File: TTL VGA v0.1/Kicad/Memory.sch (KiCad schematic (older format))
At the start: 16 parts, among them U10 UM61512A, U11 74LS245, U12 74LS374, U13 74LS245, U14 74LS245, U6 G22V10, U7 G22V10, U8 74LS139, U9 UM61512A

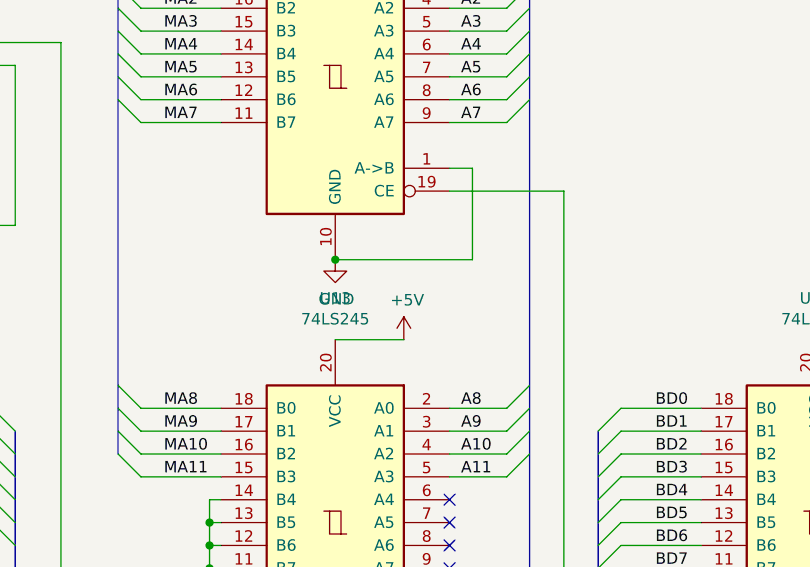
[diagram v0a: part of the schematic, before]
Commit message: update kicad
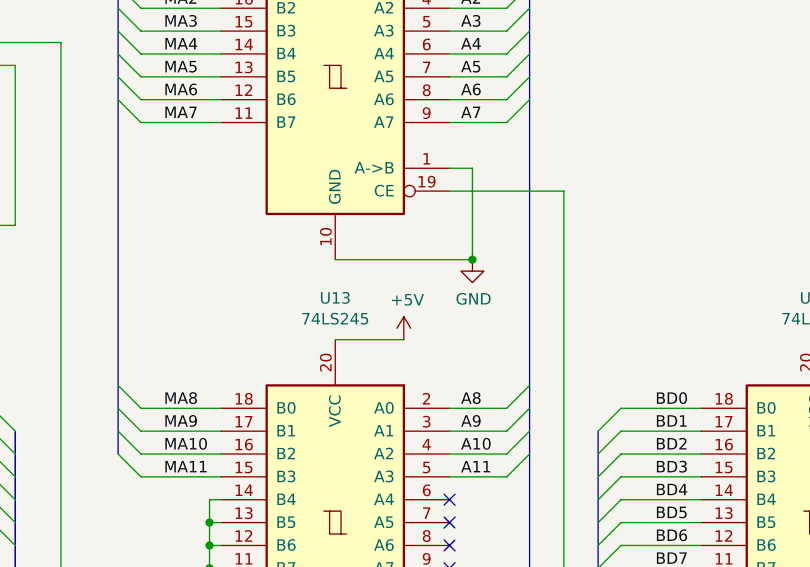
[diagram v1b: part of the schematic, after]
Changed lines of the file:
@@
 L power:GND #PWR022
 U 1 1 5E68F558
-P 4350 5750
-F 0 "#PWR022" H 4350 5500 50  0001 C CNN
-F 1 "GND" H 4355 5577 50  0000 C CNN
-F 2 "" H 4350 5750 50  0001 C CNN
-F 3 "" H 4350 5750 50  0001 C CNN
-	1    4350 5750
+P 4950 5750
+F 0 "#PWR022" H 4950 5500 50  0001 C CNN
+F 1 "GND" H 4955 5577 50  0000 C CNN
+F 2 "" H 4950 5750 50  0001 C CNN
+F 3 "" H 4950 5750 50  0001 C CNN
+	1    4950 5750
 	1    0    0    -1
 $EndComp
@@
 Wire Wire Line
 	4950 5750 4350 5750
-Connection ~ 4350 5750
 Wire Wire Line
 	4850 7300 4950 7300
@@
 $EndComp
 NoConn ~ 2600 7100
-Wire Bus Line
-	2950 6500 2950 8100
-Wire Bus Line
-	11700 2650 11700 4000
-Wire Bus Line
-	7350 5900 7350 7000
-Wire Bus Line
-	5500 6500 5500 8250
-Wire Bus Line
-	1250 4950 1250 8250
-Wire Bus Line
-	9250 2650 9250 5900
-Wire Bus Line
-	3400 3700 3400 6600
-Wire Bus Line
-	9550 1100 9550 4600
-Wire Bus Line
-	5200 1100 5200 8100
-Wire Bus Line
-	7100 1100 7100 4600
 Text Notes 7250 1800 0    50   ~ 0
 A16 and A17 are swapped on the 74LS139.\n(but it is wired like this on the perf board)\nThis will fail when using more VRAM chips.\nFix by swapping outputs in U7 (WinCUPL).
+Wire Bus Line
+	2950 6500 2950 8100
+Wire Bus Line
+	11700 2650 11700 4000
+Wire Bus Line
+	7350 5900 7350 7000
+Wire Bus Line
+	5500 6500 5500 8250
+Wire Bus Line
+	1250 4950 1250 8250
+Wire Bus Line
+	9250 2650 9250 5900
+Wire Bus Line
+	3400 3700 3400 6600
+Wire Bus Line
+	9550 1100 9550 4600
+Wire Bus Line
+	5200 1100 5200 8100
+Wire Bus Line
+	7100 1100 7100 4600
+Connection ~ 4950 5750
 $EndSCHEMATC
